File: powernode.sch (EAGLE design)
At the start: 29 parts, among them J1 ATX24RH, X1 5566-4, X2 5566-6

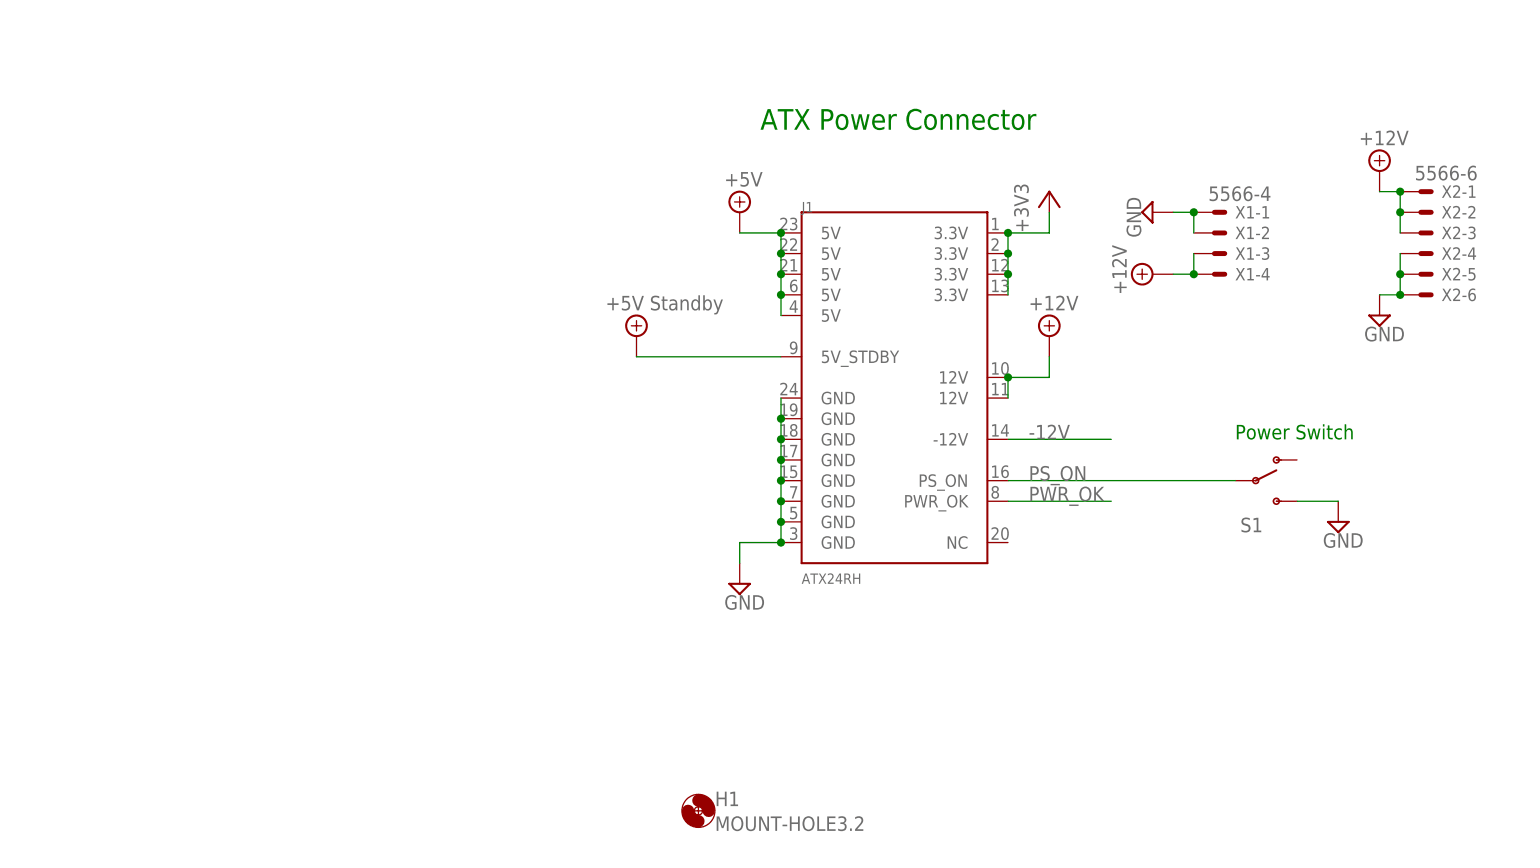
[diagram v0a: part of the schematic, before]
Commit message: working on powernode.
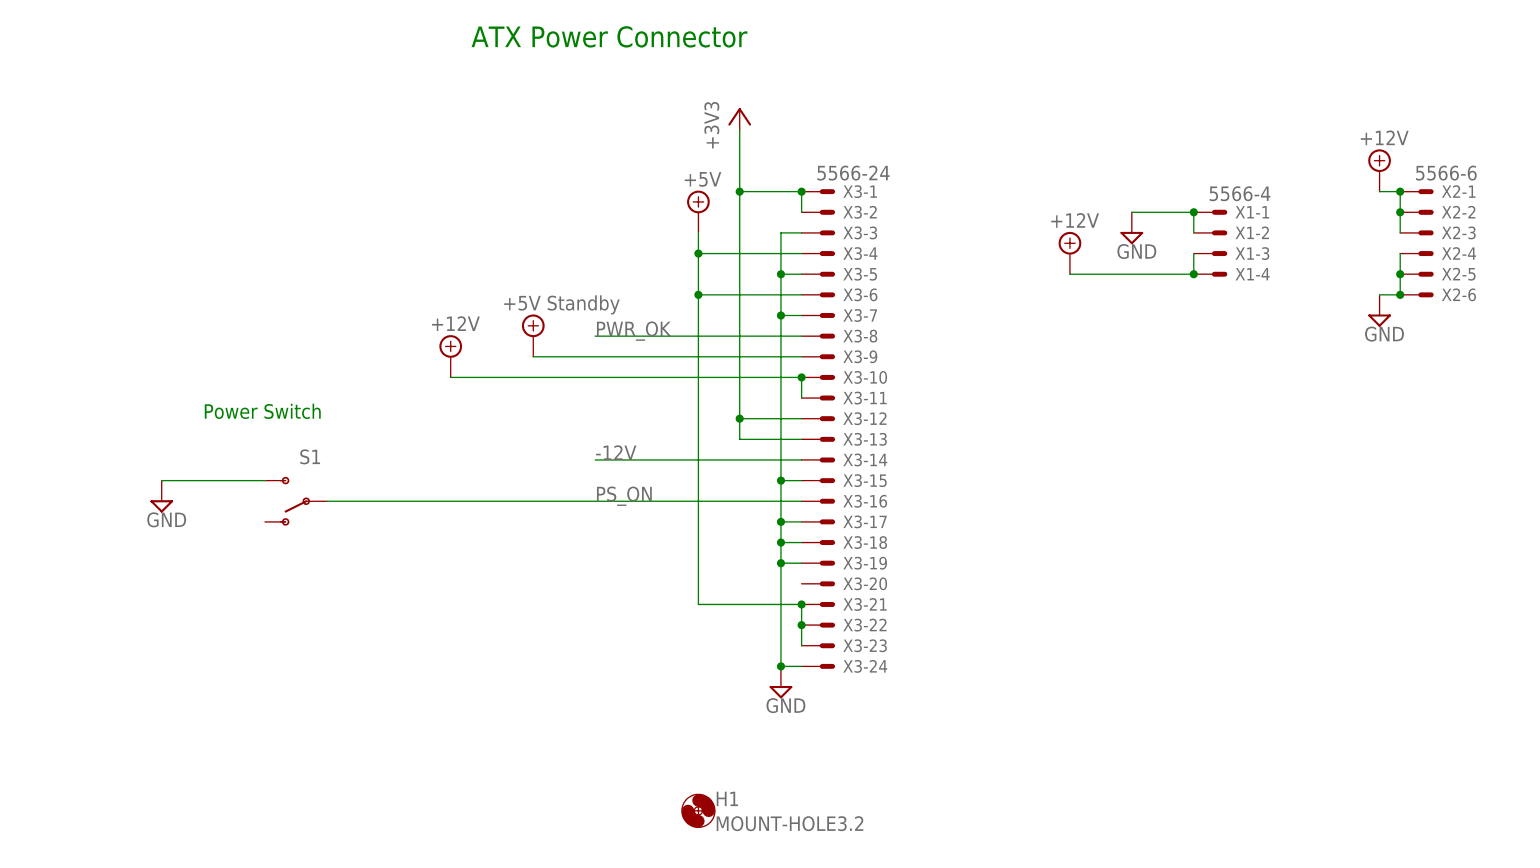
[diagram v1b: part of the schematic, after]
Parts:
- removed J1: ATX24RH, SparkFun-Connectors:ATX24RH
- added X3: 5566-24, con-molex:5566-24
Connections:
- net +12V: now also X3-10.S, X3-11.S; no longer J1.12V@0, J1.12V@1
- net +3V3: now also X3-1.S, X3-12.S, X3-13.S, X3-2.S; no longer J1.3.3V@0, J1.3.3V@1, J1.3.3V@2, J1.3.3V@3
- net +5V: now also X3-21.S, X3-22.S, X3-23.S, X3-4.S, X3-6.S; no longer J1.5V@0, J1.5V@1, J1.5V@2, J1.5V@3, J1.5V@4
- net +5V/2: now also X3-9.S; no longer J1.5V_STDBY
- net -12V: now also X3-14.S; no longer J1.-12V
- net GND: now also X3-15.S, X3-17.S, X3-18.S, X3-19.S, X3-24.S, X3-3.S, X3-5.S, X3-7.S; no longer J1.GND@0, J1.GND@1, J1.GND@2, J1.GND@3, J1.GND@4, J1.GND@5, J1.GND@6, J1.GND@7
- net PS_ON: now also X3-16.S; no longer J1.PS_ON
- net PWR_OK: now also X3-8.S; no longer J1.PWR_OK
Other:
- moved on the sheet: S1
